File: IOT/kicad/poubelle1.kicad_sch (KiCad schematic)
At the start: 3 parts

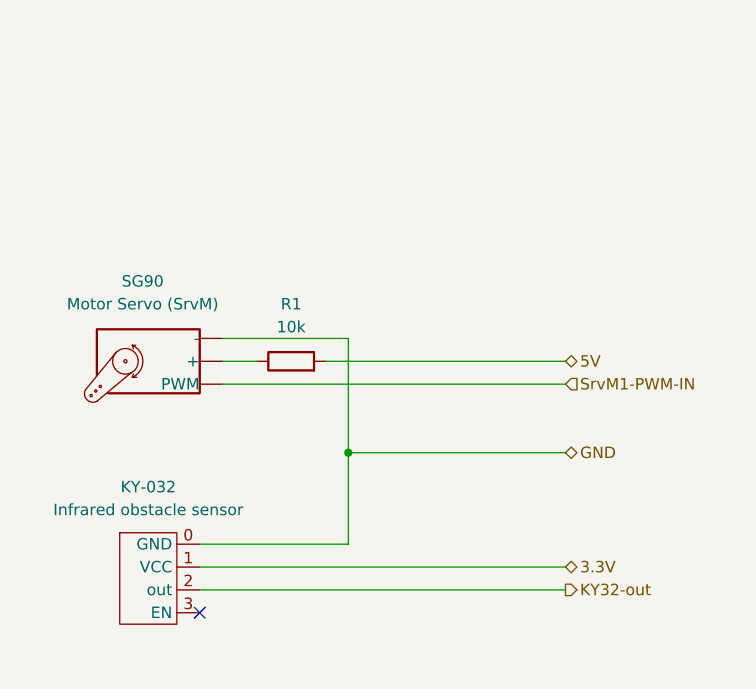
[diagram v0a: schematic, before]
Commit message: docs(iot): kicad filename + resistance + typo
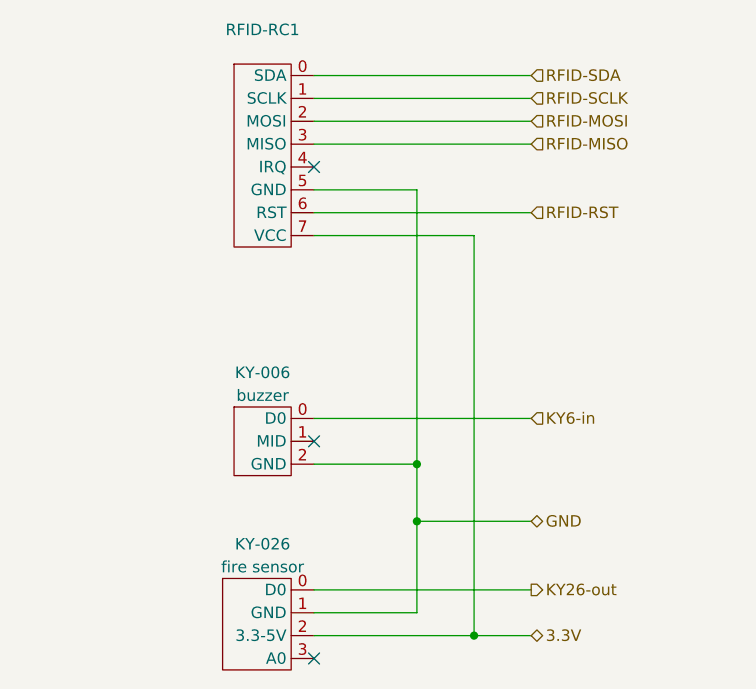
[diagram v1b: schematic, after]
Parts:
- removed KY-032: Infrared obstacle sensor, symbol OrdureX:HC-SR04
- removed R1: 10k, symbol Device:R
- removed SG90: Motor Servo (SrvM), symbol Motor:Motor_Servo
- added KY-006: buzzer, symbol OrdureX:KY-006
- added KY-026: fire sensor, symbol OrdureX:KY-026
- added RFID-RC1: ~, symbol OrdureX:RFID-RC522
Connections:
- net 3.3V: now also KY-026.2 (3.3-5V), RFID-RC1.7 (VCC)
- net GND: now also KY-006.2 (GND), KY-026.1 (GND), RFID-RC1.5 (GND)
- new net KY26-out: KY-026.0 (D0)
- new net KY6-in: KY-006.0 (D0)
- new net RFID-MISO: RFID-RC1.3 (MISO)
- new net RFID-MOSI: RFID-RC1.2 (MOSI)
- new net RFID-RST: RFID-RC1.6 (RST)
- new net RFID-SCLK: RFID-RC1.1 (SCLK)
- new net RFID-SDA: RFID-RC1.0 (SDA)
- no-connect marks 1 -> 3
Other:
- title: Poubelle 0 -> Poubelle 1
